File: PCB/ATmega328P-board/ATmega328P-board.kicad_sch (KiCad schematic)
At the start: 28 parts, among them J1 Jack-DC, J2 Headers, J3 Headers, J4 Headers, J5 Headers, J6 Conn_02x03_Odd_Even, J7 Power Screw Terminal, SW1 SW_Push, U1 ATmega328-P, U3 AMS1117, U4 AMS1117, Y1 16MHz

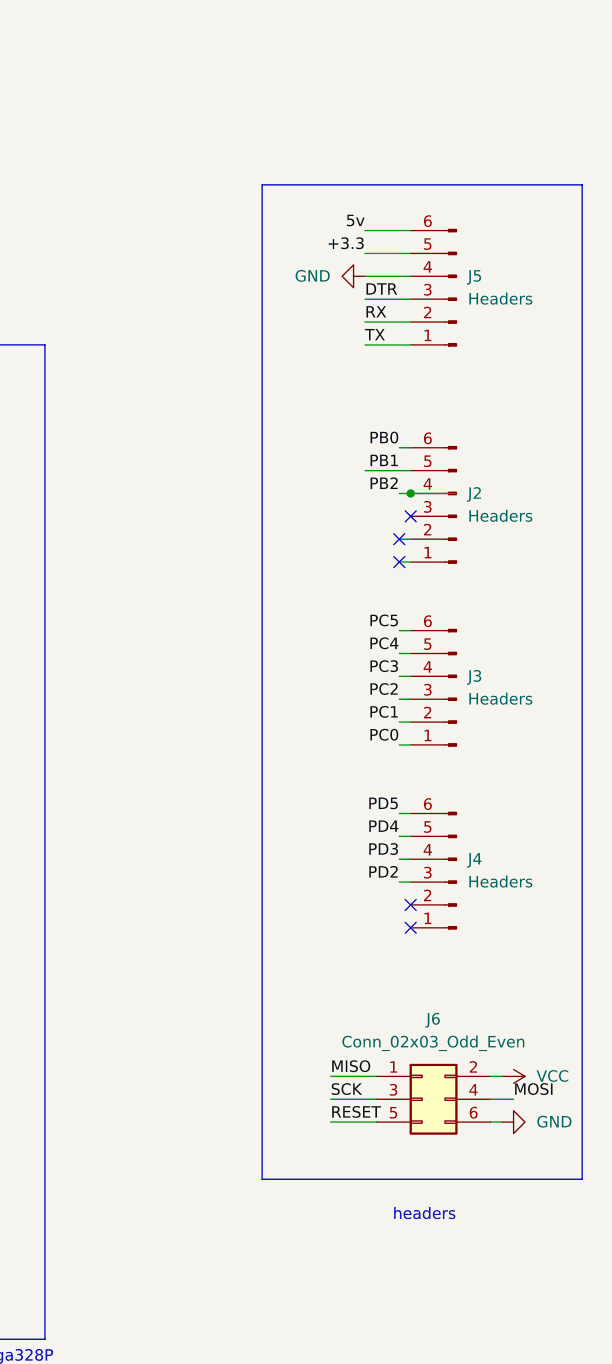
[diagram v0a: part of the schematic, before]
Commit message: Work
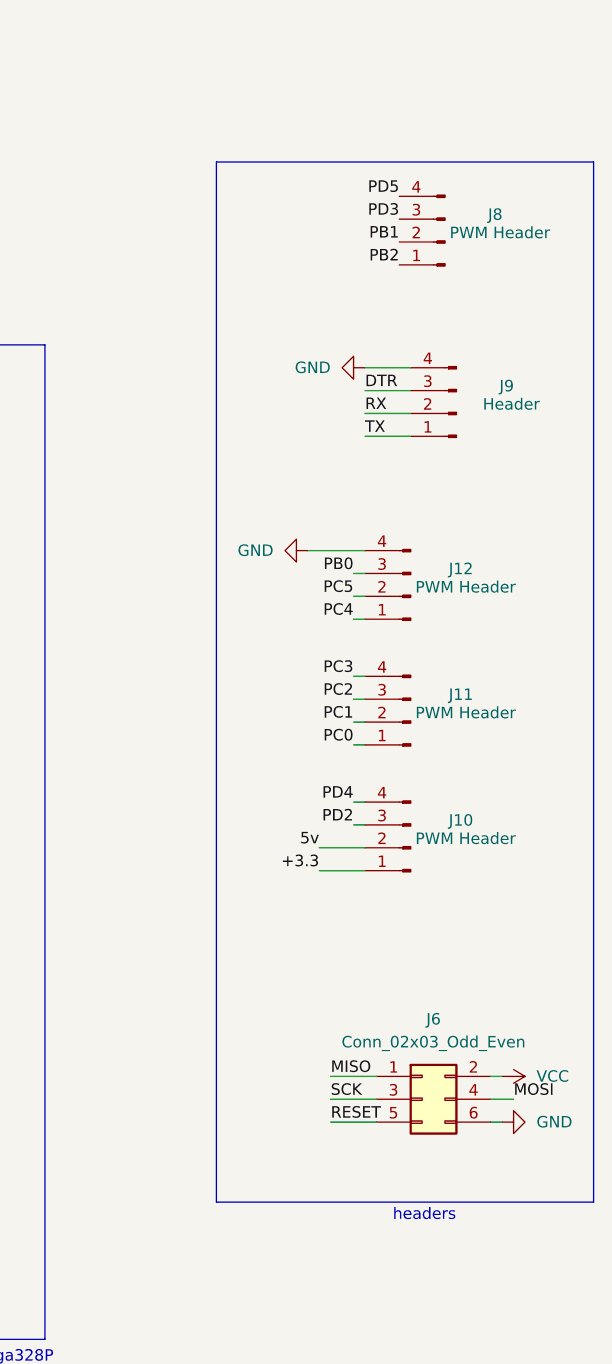
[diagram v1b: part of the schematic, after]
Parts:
- removed J2, J3, J4, J5: Headers, Connector_PinHeader_2.54mm:PinHeader_1x06_P2.54mm_Vertical, symbol Connector:Conn_01x06_Pin
- added J10, J11, J12, J8: PWM Header, Connector_PinHeader_2.54mm:PinHeader_1x04_P2.54mm_Vertical, symbol Connector:Conn_01x04_Pin
- added J9: Header, Connector_PinHeader_2.54mm:PinHeader_1x04_P2.54mm_Vertical, symbol Connector:Conn_01x04_Pin
- C1: footprint Capacitor_THT:CP_Radial_D5.0mm_P2.00mm -> Capacitor_THT:CP_Radial_D5.0mm_P2.50mm
- C3, C4, C6, C7, C8, C9: footprint Capacitor_THT:C_Disc_D5.0mm_W2.5mm_P5.00mm -> Capacitor_SMD:C_0805_2012Metric
- J7: footprint Connector_Phoenix_SPT:PhoenixContact_SPT_1.5_3-H-3.5_1x03_P3.5mm_Horizontal -> TerminalBlock_Altech:Altech_AK100_1x03_P5.00mm
- R1, R2, R3: footprint Resistor_THT:R_Axial_DIN0204_L3.6mm_D1.6mm_P7.62mm_Horizontal -> Resistor_SMD:R_0805_2012Metric
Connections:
- net +3.3: now also J10.1 (Pin_1)
- net DTR: now also J9.3 (Pin_3)
- net GND: now also J12.4 (Pin_4), J9.4 (Pin_4)
- net PB0: now also J12.3 (Pin_3)
- net PB1: now also J8.2 (Pin_2)
- net PB2: now also J8.1 (Pin_1)
- net PC0: now also J11.1 (Pin_1)
- net PC1: now also J11.2 (Pin_2)
- net PC2: now also J11.3 (Pin_3)
- net PC3: now also J11.4 (Pin_4)
- net PC4: now also J12.1 (Pin_1)
- net PC5: now also J12.2 (Pin_2)
- net PD2: now also J10.3 (Pin_3)
- net PD3: now also J8.3 (Pin_3)
- net PD4: now also J10.4 (Pin_4)
- net PD5: now also J8.4 (Pin_4)
- net RX: now also J9.2 (Pin_2)
- net TX: now also J9.1 (Pin_1)
- net VCC: now also J10.2 (Pin_2)
- no-connect marks 9 -> 4
